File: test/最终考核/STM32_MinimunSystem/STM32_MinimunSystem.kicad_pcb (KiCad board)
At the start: 2 copper layers, 96.5 x 111.8 mm, 51 parts, among them J1 USB_C_Receptacle_USB2.0, J2 Conn_01x04, J3 Conn_01x02, J4 Conn_01x19, J5 Conn_01x20, J6 Conn_01x02, J7 Conn_01x03, Q1 Q_PMOS_DGS, SW1 SW_Push, SW2 SW_Push, SW3 SW_Push, SW4 SW_Push, U1 HX9193, U2 CH340E, U3 TJA1051T-3, U4 STM32F103C8Tx, U5 AD8400ARZ50, Y1 Crystal_GND24

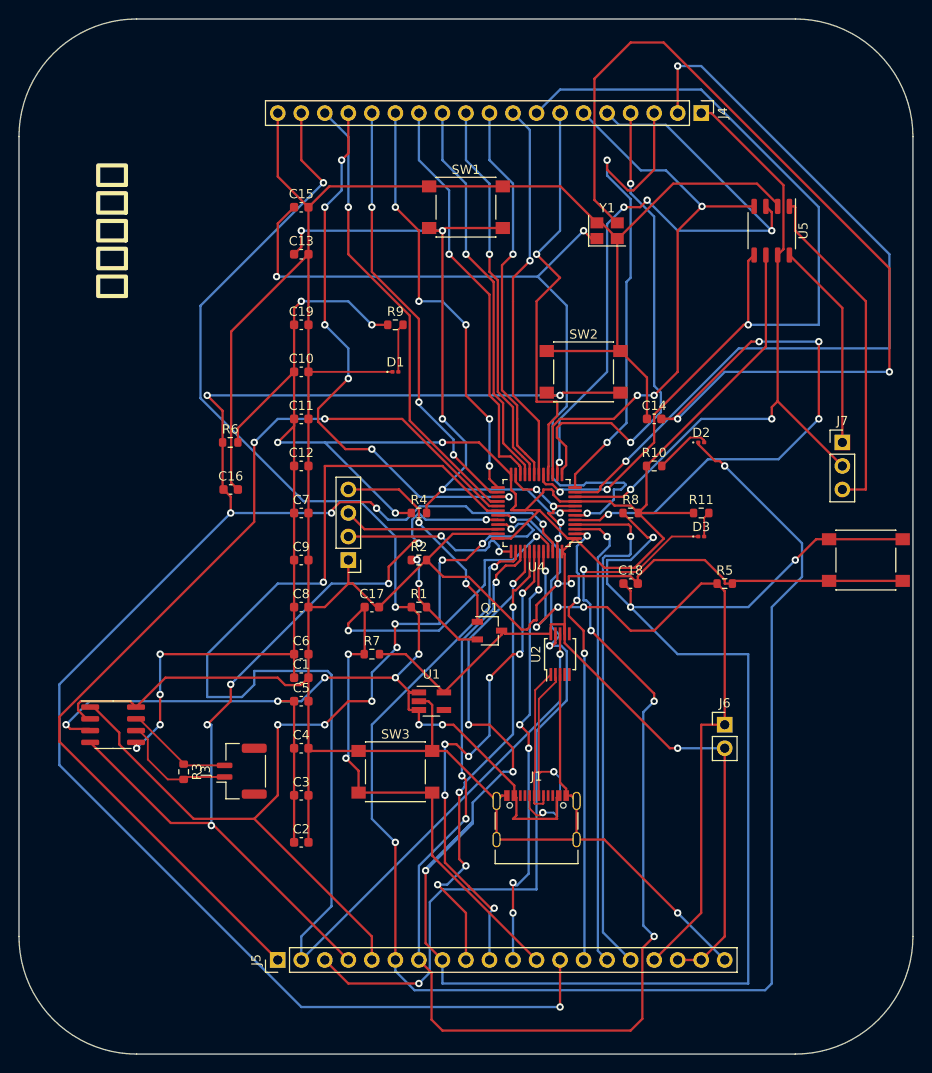
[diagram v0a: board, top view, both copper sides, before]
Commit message: 7
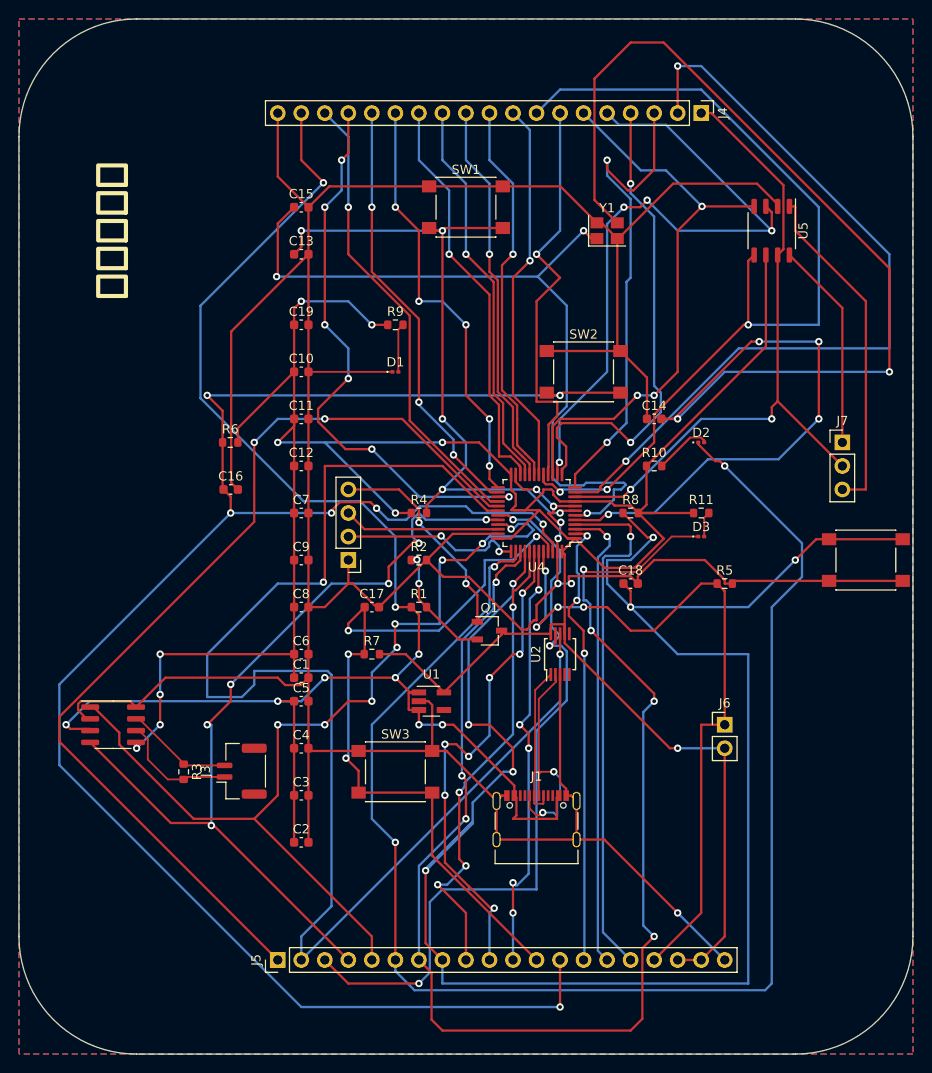
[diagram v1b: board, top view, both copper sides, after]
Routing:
- added copper zone on B.Cu, net (none)
- added copper zone on F.Cu, net (none)
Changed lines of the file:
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@@
   (segment (start 166.915 95.629122) (end 166.915 108.1295) (width 0.25) (layer "B.Cu") (net 61))
   (segment (start 165.1 129.54) (end 165.1 134.62) (width 0.25) (layer "B.Cu") (net 61))
+  (zone (net 0) (net_name "") (layer "F.Cu") (hatch edge 0.508)
+    (connect_pads (clearance 0.508))
+    (min_thickness 0.254) (filled_areas_thickness no)
+    (fill yes (thermal_gap 0.508) (thermal_bridge_width 0.508))
+    (polygon
+      (pts
+        (xy 208.28 144.78)
+        (xy 111.76 144.78)
+        (xy 111.76 33.02)
+        (xy 208.28 33.02)
+      )
+    )
+  )
+  (zone (net 0) (net_name "") (layer "B.Cu") (hatch edge 0.508)
+    (connect_pads (clearance 0.508))
+    (min_thickness 0.254) (filled_areas_thickness no)
+    (fill yes (thermal_gap 0.508) (thermal_bridge_width 0.508))
+    (polygon
+      (pts
+        (xy 208.28 144.78)
+        (xy 111.76 144.78)
+        (xy 111.76 33.02)
+        (xy 208.28 33.02)
+      )
+    )
+  )
 )
